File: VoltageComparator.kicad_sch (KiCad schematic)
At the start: 6 parts, among them U18 LM358, U5 74LS08

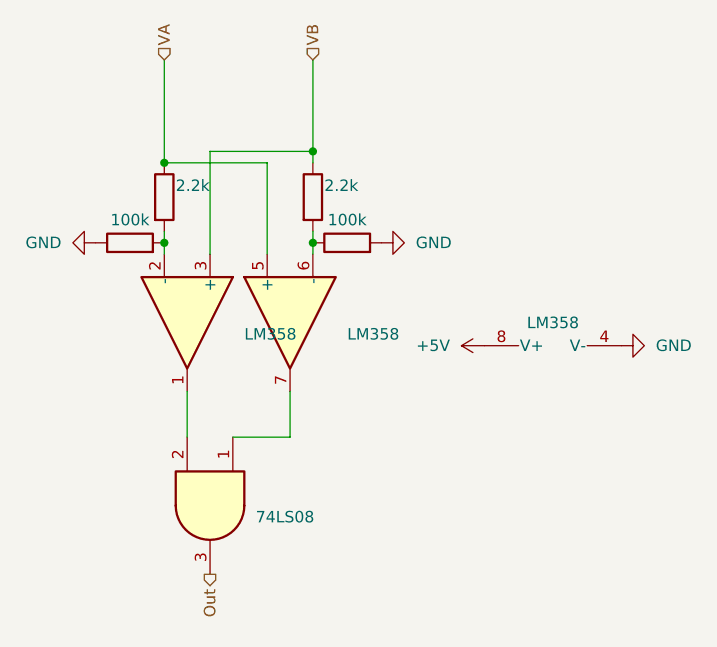
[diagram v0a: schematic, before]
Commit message: Started PCB Work
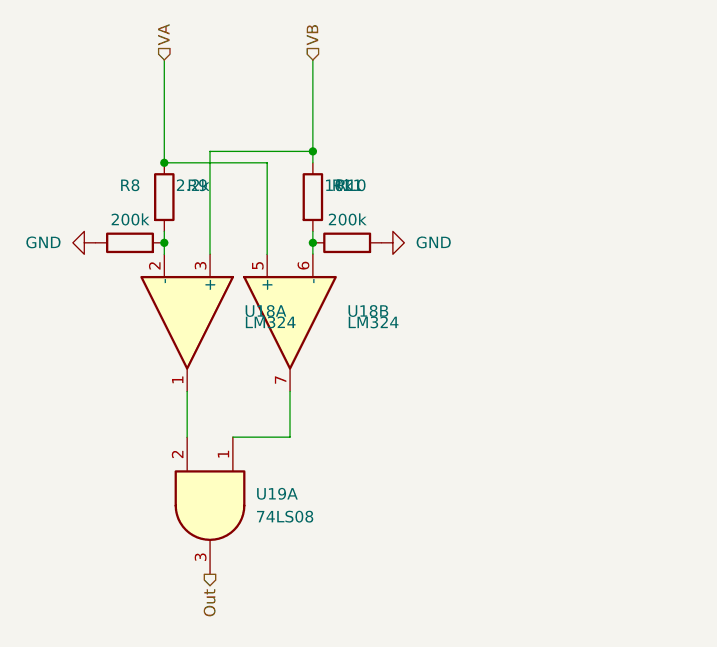
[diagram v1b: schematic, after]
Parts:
- removed unit 3 of U18
- R10: renamed from R7; value 2.2k -> 10k; footprint (none) -> Resistor_SMD:R_0805_2012Metric_Pad1.20x1.40mm_HandSolder
- R11: renamed from R8; value 100k -> 200k; footprint (none) -> Resistor_SMD:R_0805_2012Metric_Pad1.20x1.40mm_HandSolder
- R8: renamed from R5; value 100k -> 200k; footprint (none) -> Resistor_SMD:R_0805_2012Metric_Pad1.20x1.40mm_HandSolder
- R9: renamed from R6; footprint (none) -> Resistor_SMD:R_0805_2012Metric_Pad1.20x1.40mm_HandSolder
- U18: value LM358 -> LM324; footprint (none) -> Package_SO:SOIC-14_3.9x8.7mm_P1.27mm; symbol Amplifier_Operational:LM358 -> Amplifier_Operational:LM324
- U19: renamed from U5; footprint (none) -> Package_SO:SOIC-14_3.9x8.7mm_P1.27mm

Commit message: routed
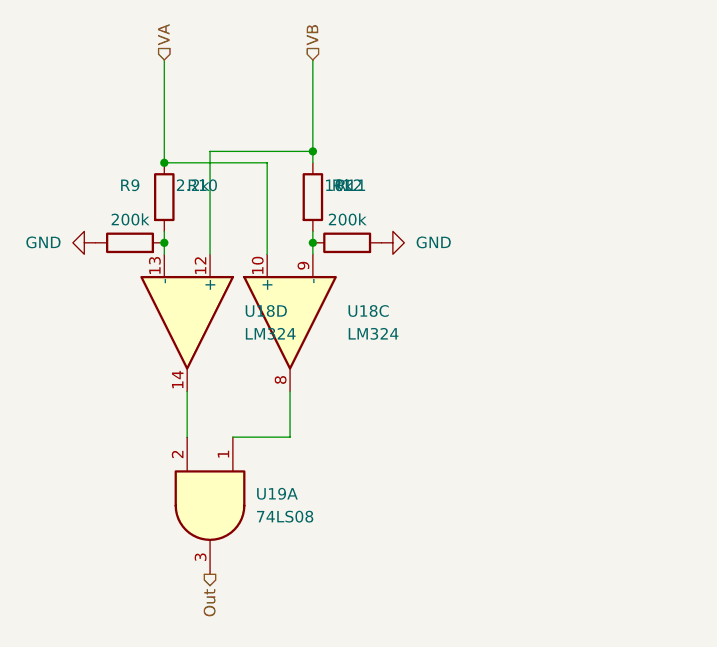
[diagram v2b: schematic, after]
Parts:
- renumbered R9 to R10, R10 to R11, R11 to R12, R8 to R9
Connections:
- net VA: now also U18.10 (+); no longer U18.5 (+)
- net VB: now also U18.12 (+); no longer U18.3 (+)
- net at U19.1: now also U18.8; no longer U18.7
- net at U19.2: now also U18.14; no longer U18.1
- net at R10.2, R9.2: now also U18.13 (-); no longer U18.2 (-)
- net at R11.2, R12.1: now also U18.9 (-); no longer U18.6 (-)
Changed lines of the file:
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@@
 		(on_board yes)
 		(dnp no)
-		(fields_autoplaced yes)
 		(property "Reference" "U19"
 			(at 58.42 95.2416 90)
@@
 		(dnp no)
 		(fields_autoplaced yes)
-		(property "Reference" "#PWR087"
+		(property "Reference" "#PWR088"
 			(at 78.74 67.31 0)
 			(effects
@@
 			(project "ECE145Mastermind"
 				(path "/8c64fe8a-5d6b-41bc-b3a3-9bda7b2e0f2c/218d925b-79f6-474b-97b2-c0ad78559cda"
-					(reference "#PWR091")
-					(unit 1)
-				)
-				(path "/8c64fe8a-5d6b-41bc-b3a3-9bda7b2e0f2c/4f59e726-7fd4-4ef0-8dbb-7a41976aa953"
-					(reference "#PWR087")
-					(unit 1)
-				)
-				(path "/8c64fe8a-5d6b-41bc-b3a3-9bda7b2e0f2c/acb554fe-df67-46ea-bc1c-079edbbfc216"
-					(reference "#PWR089")
-					(unit 1)
-				)
-				(path "/8c64fe8a-5d6b-41bc-b3a3-9bda7b2e0f2c/d4674d5d-47f2-4c8d-9fae-4e866cda3652"
-					(reference "#PWR093")
+					(reference "#PWR092")
+					(unit 1)
+				)
+				(path "/8c64fe8a-5d6b-41bc-b3a3-9bda7b2e0f2c/4f59e726-7fd4-4ef0-8dbb-7a41976aa953"
+					(reference "#PWR088")
+					(unit 1)
+				)
+				(path "/8c64fe8a-5d6b-41bc-b3a3-9bda7b2e0f2c/acb554fe-df67-46ea-bc1c-079edbbfc216"
+					(reference "#PWR090")
+					(unit 1)
+				)
+				(path "/8c64fe8a-5d6b-41bc-b3a3-9bda7b2e0f2c/d4674d5d-47f2-4c8d-9fae-4e866cda3652"
+					(reference "#PWR094")
 					(unit 1)
 				)
@@
 		(on_board yes)
 		(dnp no)
-		(property "Reference" "R9"
+		(property "Reference" "R10"
 			(at 50.8 60.9599 0)
 			(effects
@@
 			(project "ECE145Mastermind"
 				(path "/8c64fe8a-5d6b-41bc-b3a3-9bda7b2e0f2c/218d925b-79f6-474b-97b2-c0ad78559cda"
-					(reference "R17")
-					(unit 1)
-				)
-				(path "/8c64fe8a-5d6b-41bc-b3a3-9bda7b2e0f2c/4f59e726-7fd4-4ef0-8dbb-7a41976aa953"
-					(reference "R9")
-					(unit 1)
-				)
-				(path "/8c64fe8a-5d6b-41bc-b3a3-9bda7b2e0f2c/acb554fe-df67-46ea-bc1c-079edbbfc216"
-					(reference "R13")
-					(unit 1)
-				)
-				(path "/8c64fe8a-5d6b-41bc-b3a3-9bda7b2e0f2c/d4674d5d-47f2-4c8d-9fae-4e866cda3652"
-					(reference "R21")
+					(reference "R18")
+					(unit 1)
+				)
+				(path "/8c64fe8a-5d6b-41bc-b3a3-9bda7b2e0f2c/4f59e726-7fd4-4ef0-8dbb-7a41976aa953"
+					(reference "R10")
+					(unit 1)
+				)
+				(path "/8c64fe8a-5d6b-41bc-b3a3-9bda7b2e0f2c/acb554fe-df67-46ea-bc1c-079edbbfc216"
+					(reference "R14")
+					(unit 1)
+				)
+				(path "/8c64fe8a-5d6b-41bc-b3a3-9bda7b2e0f2c/d4674d5d-47f2-4c8d-9fae-4e866cda3652"
+					(reference "R22")
 					(unit 1)
 				)
@@
 		(dnp no)
 		(fields_autoplaced yes)
-		(property "Reference" "#PWR086"
+		(property "Reference" "#PWR087"
 			(at 34.29 67.31 0)
 			(effects
@@
 			(project "ECE145Mastermind"
 				(path "/8c64fe8a-5d6b-41bc-b3a3-9bda7b2e0f2c/218d925b-79f6-474b-97b2-c0ad78559cda"
-					(reference "#PWR090")
-					(unit 1)
-				)
-				(path "/8c64fe8a-5d6b-41bc-b3a3-9bda7b2e0f2c/4f59e726-7fd4-4ef0-8dbb-7a41976aa953"
-					(reference "#PWR086")
-					(unit 1)
-				)
-				(path "/8c64fe8a-5d6b-41bc-b3a3-9bda7b2e0f2c/acb554fe-df67-46ea-bc1c-079edbbfc216"
-					(reference "#PWR088")
-					(unit 1)
-				)
-				(path "/8c64fe8a-5d6b-41bc-b3a3-9bda7b2e0f2c/d4674d5d-47f2-4c8d-9fae-4e866cda3652"
-					(reference "#PWR092")
+					(reference "#PWR091")
+					(unit 1)
+				)
+				(path "/8c64fe8a-5d6b-41bc-b3a3-9bda7b2e0f2c/4f59e726-7fd4-4ef0-8dbb-7a41976aa953"
+					(reference "#PWR087")
+					(unit 1)
+				)
+				(path "/8c64fe8a-5d6b-41bc-b3a3-9bda7b2e0f2c/acb554fe-df67-46ea-bc1c-079edbbfc216"
+					(reference "#PWR089")
+					(unit 1)
+				)
+				(path "/8c64fe8a-5d6b-41bc-b3a3-9bda7b2e0f2c/d4674d5d-47f2-4c8d-9fae-4e866cda3652"
+					(reference "#PWR093")
 					(unit 1)
 				)
@@
 		(on_board yes)
 		(dnp no)
-		(property "Reference" "R10"
+		(property "Reference" "R11"
 			(at 67.31 60.9599 0)
 			(effects
@@
 			(project "ECE145Mastermind"
 				(path "/8c64fe8a-5d6b-41bc-b3a3-9bda7b2e0f2c/218d925b-79f6-474b-97b2-c0ad78559cda"
-					(reference "R18")
-					(unit 1)
-				)
-				(path "/8c64fe8a-5d6b-41bc-b3a3-9bda7b2e0f2c/4f59e726-7fd4-4ef0-8dbb-7a41976aa953"
-					(reference "R10")
-					(unit 1)
-				)
-				(path "/8c64fe8a-5d6b-41bc-b3a3-9bda7b2e0f2c/acb554fe-df67-46ea-bc1c-079edbbfc216"
-					(reference "R14")
-					(unit 1)
-				)
-				(path "/8c64fe8a-5d6b-41bc-b3a3-9bda7b2e0f2c/d4674d5d-47f2-4c8d-9fae-4e866cda3652"
-					(reference "R22")
+					(reference "R19")
+					(unit 1)
+				)
+				(path "/8c64fe8a-5d6b-41bc-b3a3-9bda7b2e0f2c/4f59e726-7fd4-4ef0-8dbb-7a41976aa953"
+					(reference "R11")
+					(unit 1)
+				)
+				(path "/8c64fe8a-5d6b-41bc-b3a3-9bda7b2e0f2c/acb554fe-df67-46ea-bc1c-079edbbfc216"
+					(reference "R15")
+					(unit 1)
+				)
+				(path "/8c64fe8a-5d6b-41bc-b3a3-9bda7b2e0f2c/d4674d5d-47f2-4c8d-9fae-4e866cda3652"
+					(reference "R23")
 					(unit 1)
 				)
@@
 		(at 62.23 76.2 90)
 		(mirror x)
-		(unit 2)
+		(unit 3)
 		(exclude_from_sim no)
 		(in_bom yes)
@@
 		)
 		(property "Value" "LM324"
-			(at 68.58 76.1999 90)
+			(at 68.58 77.4699 90)
 			(effects
 				(font
@@
 				(path "/8c64fe8a-5d6b-41bc-b3a3-9bda7b2e0f2c/4f59e726-7fd4-4ef0-8dbb-7a41976aa953"
 					(reference "U18")
+					(unit 3)
+				)
+				(path "/8c64fe8a-5d6b-41bc-b3a3-9bda7b2e0f2c/acb554fe-df67-46ea-bc1c-079edbbfc216"
+					(reference "U18")
 					(unit 2)
-				)
-				(path "/8c64fe8a-5d6b-41bc-b3a3-9bda7b2e0f2c/acb554fe-df67-46ea-bc1c-079edbbfc216"
-					(reference "U18")
-					(unit 4)
 				)
 				(path "/8c64fe8a-5d6b-41bc-b3a3-9bda7b2e0f2c/d4674d5d-47f2-4c8d-9fae-4e866cda3652"
@@
 		(lib_id "Amplifier_Operational:LM324")
 		(at 50.8 76.2 270)
-		(unit 1)
+		(unit 4)
 		(exclude_from_sim no)
 		(in_bom yes)
@@
 		)
 		(property "Value" "LM324"
-			(at 57.15 76.1999 90)
+			(at 57.15 77.4699 90)
 			(effects
 				(font
@@
 				(path "/8c64fe8a-5d6b-41bc-b3a3-9bda7b2e0f2c/4f59e726-7fd4-4ef0-8dbb-7a41976aa953"
 					(reference "U18")
-					(unit 1)
+					(unit 4)
 				)
 				(path "/8c64fe8a-5d6b-41bc-b3a3-9bda7b2e0f2c/acb554fe-df67-46ea-bc1c-079edbbfc216"
 					(reference "U18")
-					(unit 3)
+					(unit 1)
 				)
 				(path "/8c64fe8a-5d6b-41bc-b3a3-9bda7b2e0f2c/d4674d5d-47f2-4c8d-9fae-4e866cda3652"
@@
 		(on_board yes)
 		(dnp no)
-		(property "Reference" "R8"
+		(property "Reference" "R9"
 			(at 44.45 60.96 90)
 			(effects
@@
 			(project "ECE145Mastermind"
 				(path "/8c64fe8a-5d6b-41bc-b3a3-9bda7b2e0f2c/218d925b-79f6-474b-97b2-c0ad78559cda"
-					(reference "R16")
-					(unit 1)
-				)
-				(path "/8c64fe8a-5d6b-41bc-b3a3-9bda7b2e0f2c/4f59e726-7fd4-4ef0-8dbb-7a41976aa953"
-					(reference "R8")
-					(unit 1)
-				)
-				(path "/8c64fe8a-5d6b-41bc-b3a3-9bda7b2e0f2c/acb554fe-df67-46ea-bc1c-079edbbfc216"
-					(reference "R12")
-					(unit 1)
-				)
-				(path "/8c64fe8a-5d6b-41bc-b3a3-9bda7b2e0f2c/d4674d5d-47f2-4c8d-9fae-4e866cda3652"
-					(reference "R20")
+					(reference "R17")
+					(unit 1)
+				)
+				(path "/8c64fe8a-5d6b-41bc-b3a3-9bda7b2e0f2c/4f59e726-7fd4-4ef0-8dbb-7a41976aa953"
+					(reference "R9")
+					(unit 1)
+				)
+				(path "/8c64fe8a-5d6b-41bc-b3a3-9bda7b2e0f2c/acb554fe-df67-46ea-bc1c-079edbbfc216"
+					(reference "R13")
+					(unit 1)
+				)
+				(path "/8c64fe8a-5d6b-41bc-b3a3-9bda7b2e0f2c/d4674d5d-47f2-4c8d-9fae-4e866cda3652"
+					(reference "R21")
 					(unit 1)
 				)
@@
 		(on_board yes)
 		(dnp no)
-		(property "Reference" "R11"
+		(property "Reference" "R12"
 			(at 68.58 60.96 90)
 			(effects
@@
 			(project "ECE145Mastermind"
 				(path "/8c64fe8a-5d6b-41bc-b3a3-9bda7b2e0f2c/218d925b-79f6-474b-97b2-c0ad78559cda"
-					(reference "R19")
-					(unit 1)
-				)
-				(path "/8c64fe8a-5d6b-41bc-b3a3-9bda7b2e0f2c/4f59e726-7fd4-4ef0-8dbb-7a41976aa953"
-					(reference "R11")
-					(unit 1)
-				)
-				(path "/8c64fe8a-5d6b-41bc-b3a3-9bda7b2e0f2c/acb554fe-df67-46ea-bc1c-079edbbfc216"
-					(reference "R15")
-					(unit 1)
-				)
-				(path "/8c64fe8a-5d6b-41bc-b3a3-9bda7b2e0f2c/d4674d5d-47f2-4c8d-9fae-4e866cda3652"
-					(reference "R23")
-					(unit 1)
-				)
+					(reference "R20")
+					(unit 1)
+				)
+				(path "/8c64fe8a-5d6b-41bc-b3a3-9bda7b2e0f2c/4f59e726-7fd4-4ef0-8dbb-7a41976aa953"
+					(reference "R12")
+					(unit 1)
+				)
+				(path "/8c64fe8a-5d6b-41bc-b3a3-9bda7b2e0f2c/acb554fe-df67-46ea-bc1c-079edbbfc216"
+					(reference "R16")
+					(unit 1)
+				)
+				(path "/8c64fe8a-5d6b-41bc-b3a3-9bda7b2e0f2c/d4674d5d-47f2-4c8d-9fae-4e866cda3652"
+					(reference "R24")
+					(unit 1)
+				)
